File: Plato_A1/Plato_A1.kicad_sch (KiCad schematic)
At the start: 23 parts, among them J1 Conn_01x03_Socket, J2 Conn_01x03_Pin

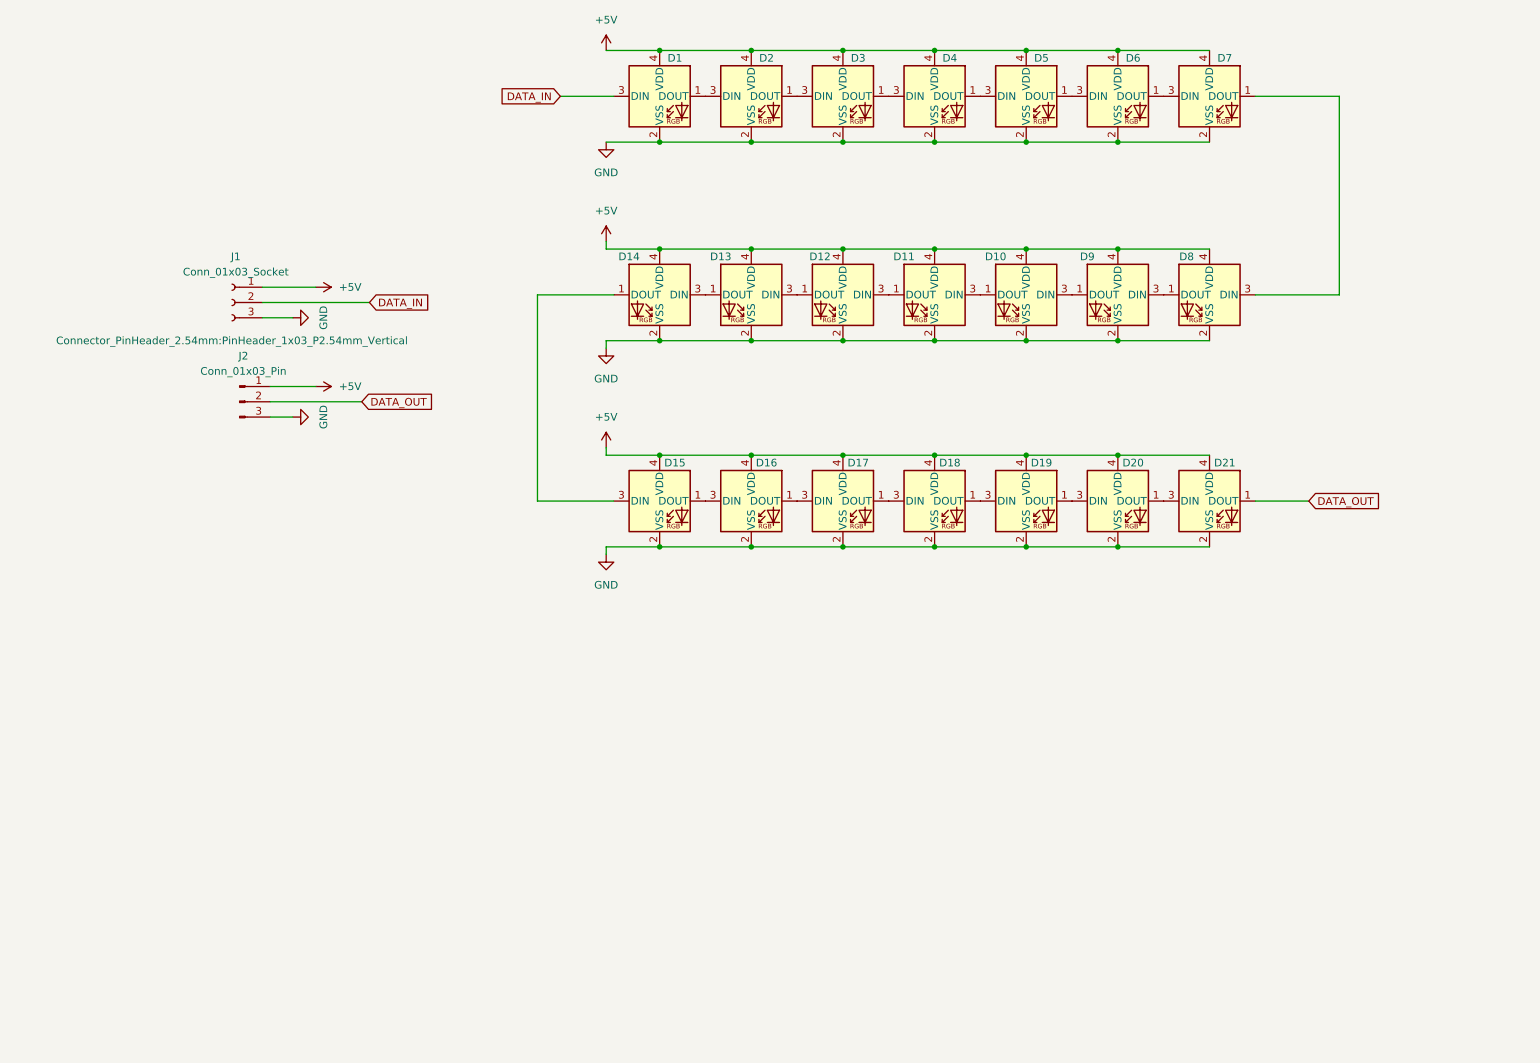
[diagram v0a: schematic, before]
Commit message: Abortative redesign
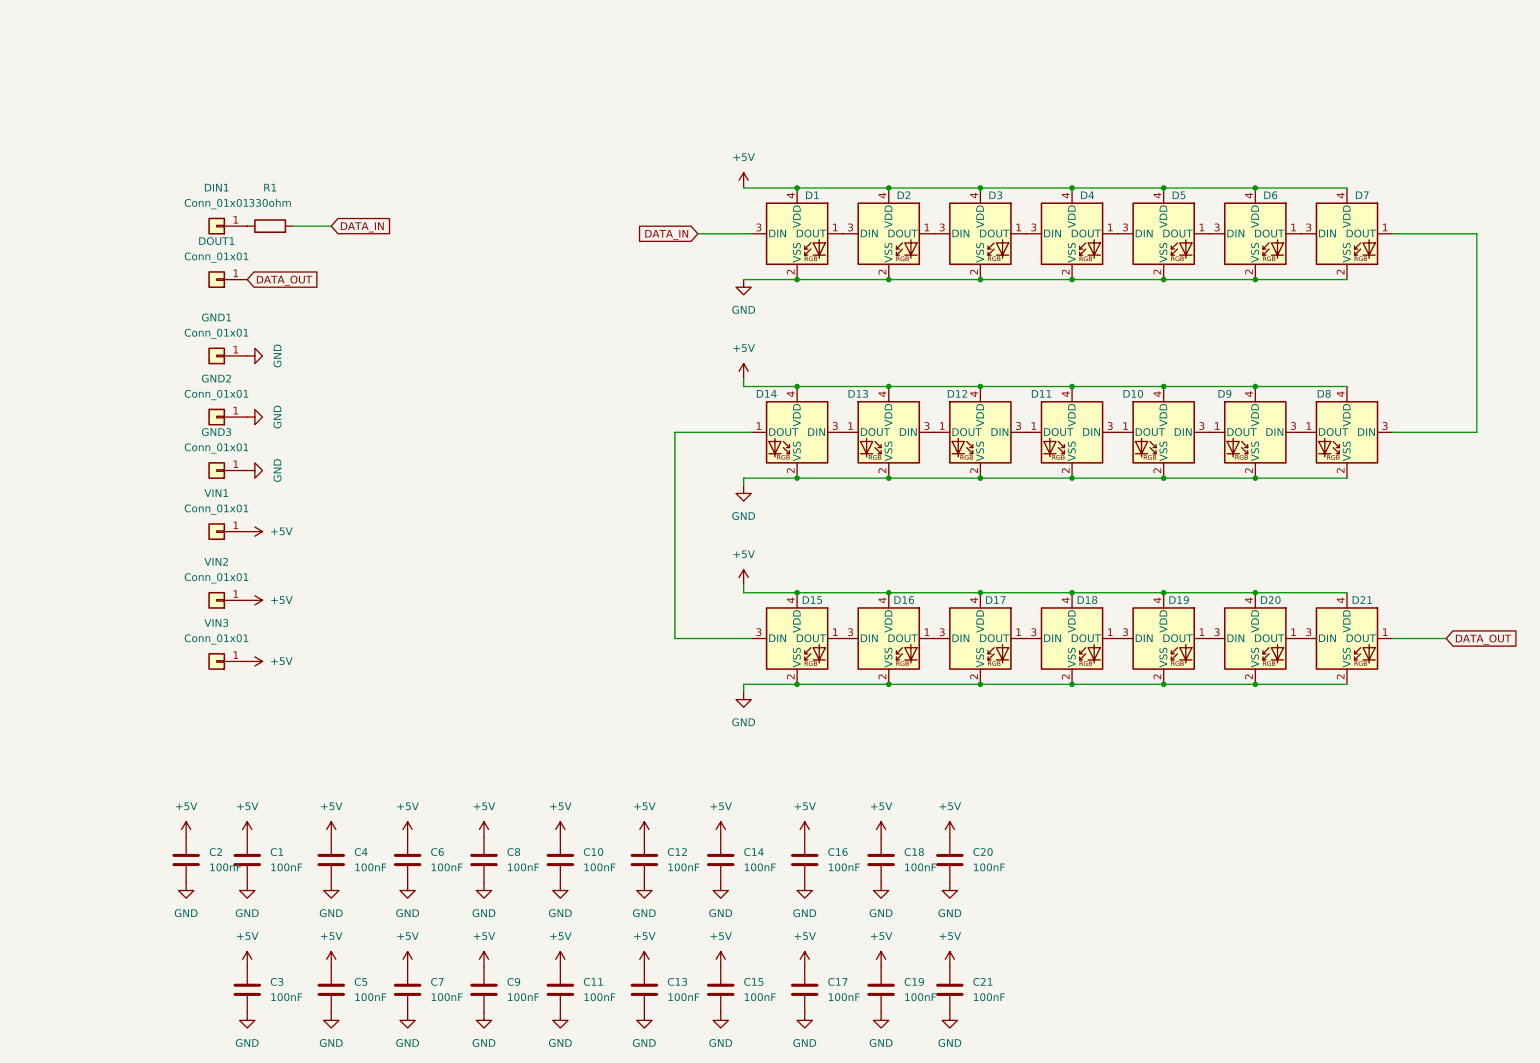
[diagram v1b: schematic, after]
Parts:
- removed J1: Conn_01x03_Socket, Connector_PinHeader_2.54mm:PinHeader_1x03_P2.54mm_Vertical, symbol Connector:Conn_01x03_Socket
- removed J2: Conn_01x03_Pin, Connector_PinHeader_2.54mm:PinHeader_1x03_P2.54mm_Vertical, symbol Connector:Conn_01x03_Pin
- added C1, C10, C11, C12, C13, C14, C15, C16, C17, C18, C19, C2, C20, C21, C3, C4, C5, C6, C7, C8, C9: 100nF, Capacitor_SMD:C_0402_1005Metric, symbol Device:C
- added DIN1, DOUT1: Conn_01x01, Library:DataHole, symbol Connector_Generic:Conn_01x01
- added GND1, GND2, GND3, VIN1, VIN2, VIN3: Conn_01x01, Library:PowerHole, symbol Connector_Generic:Conn_01x01
- added R1: 330ohm, Resistor_SMD:R_0402_1005Metric, symbol Device:R
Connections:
- net +5V: now also C1.1, C10.1, C11.1, C12.1, C13.1, C14.1, C15.1, C16.1, C17.1, C18.1, C19.1, C2.1, C20.1, C21.1, C3.1, C4.1, C5.1, C6.1, C7.1, C8.1, C9.1, VIN1.1 (Pin_1), VIN2.1 (Pin_1), VIN3.1 (Pin_1)
- net DATA_IN: now also R1.2
- net DATA_OUT: now also DOUT1.1 (Pin_1)
- net GND: now also C1.2, C10.2, C11.2, C12.2, C13.2, C14.2, C15.2, C16.2, C17.2, C18.2, C19.2, C2.2, C20.2, C21.2, C3.2, C4.2, C5.2, C6.2, C7.2, C8.2, C9.2, GND1.1 (Pin_1), GND2.1 (Pin_1), GND3.1 (Pin_1)
- new net: DIN1.1 (Pin_1), R1.1
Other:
- moved on the sheet: D1, D10, D11, D12, D13, D14, D15, D16, D17, D18, D19, D2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

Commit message: Restore final product
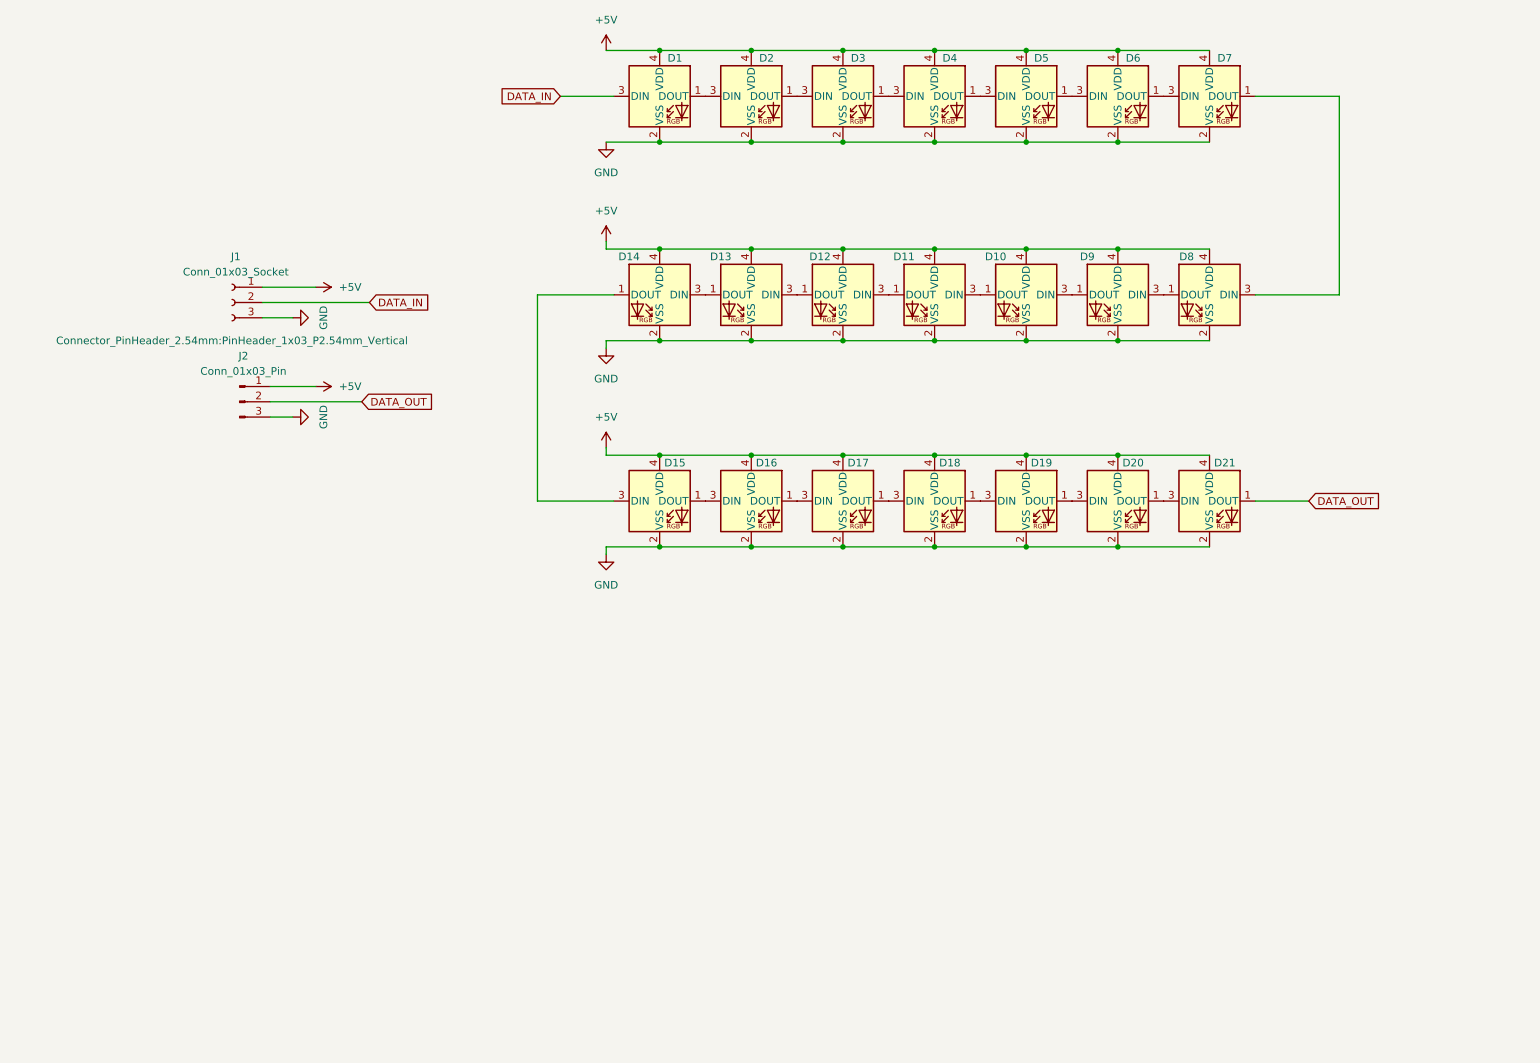
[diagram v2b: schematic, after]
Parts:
- removed C1, C10, C11, C12, C13, C14, C15, C16, C17, C18, C19, C2, C20, C21, C3, C4, C5, C6, C7, C8, C9: 100nF, Capacitor_SMD:C_0402_1005Metric, symbol Device:C
- removed DIN1, DOUT1: Conn_01x01, Library:DataHole, symbol Connector_Generic:Conn_01x01
- removed GND1, GND2, GND3, VIN1, VIN2, VIN3: Conn_01x01, Library:PowerHole, symbol Connector_Generic:Conn_01x01
- removed R1: 330ohm, Resistor_SMD:R_0402_1005Metric, symbol Device:R
- added J1: Conn_01x03_Socket, Connector_PinHeader_2.54mm:PinHeader_1x03_P2.54mm_Vertical, symbol Connector:Conn_01x03_Socket
- added J2: Conn_01x03_Pin, Connector_PinHeader_2.54mm:PinHeader_1x03_P2.54mm_Vertical, symbol Connector:Conn_01x03_Pin
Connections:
- net +5V: now also J1.1 (Pin_1), J2.1 (Pin_1)
- net DATA_IN: now also J1.2 (Pin_2)
- net DATA_OUT: now also J2.2 (Pin_2)
- net GND: now also J1.3 (Pin_3), J2.3 (Pin_3)
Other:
- moved on the sheet: D1, D10, D11, D12, D13, D14, D15, D16, D17, D18, D19, D2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
